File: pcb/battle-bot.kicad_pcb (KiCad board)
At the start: 4 copper layers, 82.1 x 54.4 mm, 229 parts, among them J1 Conn_01x01_Pin, J10 Conn_01x01_Pin, J11 Conn_01x01_Pin, J12 Conn_01x01_Pin, J13 Conn_ARM_SWD_TagConnect_TC203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, J3 Conn_01x01_Pin, J4 Conn_01x01_Pin, J5 Conn_01x01_Pin, J6 Conn_01x01_Pin, J7 Conn_01x01_Pin, J8 Conn_01x01_Pin, J9 Conn_01x01_Pin, Q1 AON7544, Q2 AO3401A, Q21 GANE3R9, Q22 GANE3R9, Q23 GANE3R9, Q24 GANE3R9, Q25 GANE3R9, Q26 GANE3R9, Q27 AON7544, Q28 AON7544, Q29 AON7544, Q30 AON7544, Q31 AON7544, Q32 AON7544, Q33 AON7544, Q34 AON7544, Q35 AON7544, Q36 AON7544, Q37 AON7544, Q38 AON7544, Q39 AON7544, Q40 AON7544, Q41 AON7544, Q42 AON7544, Q43 AON7544, U1 TPS53319, U10 LMG1205, U11 LMG1205, U12 LMG1205, U13 ACS780xLRTR-100B, U15 LP38690SD, U2 nRF24L01P, U3 AT2401C, U4 ICM-42688-P, U6 STM32G431RBTx, U7 DRV8323H, U8 DRV8323H, U9 DRV8323H, Y1 16MHz, Y2 16MHz

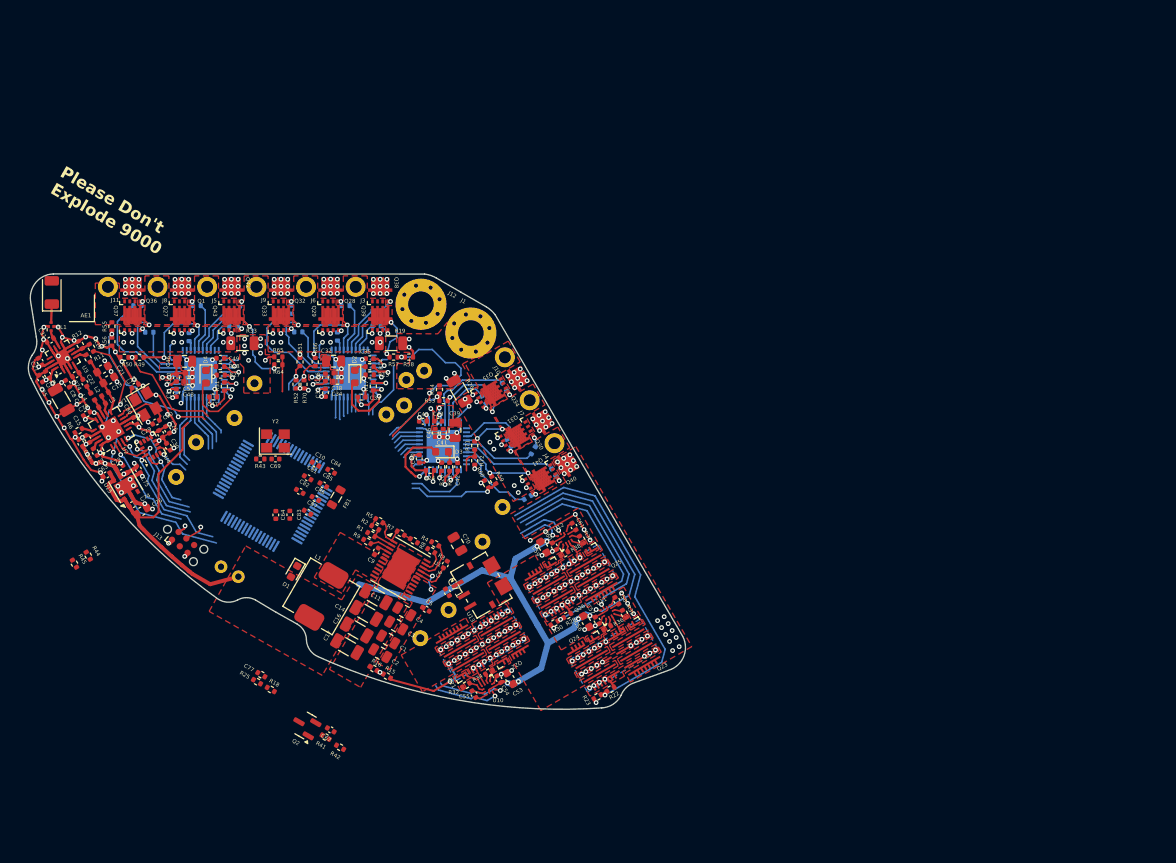
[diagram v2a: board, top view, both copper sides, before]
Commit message: Finish pcb
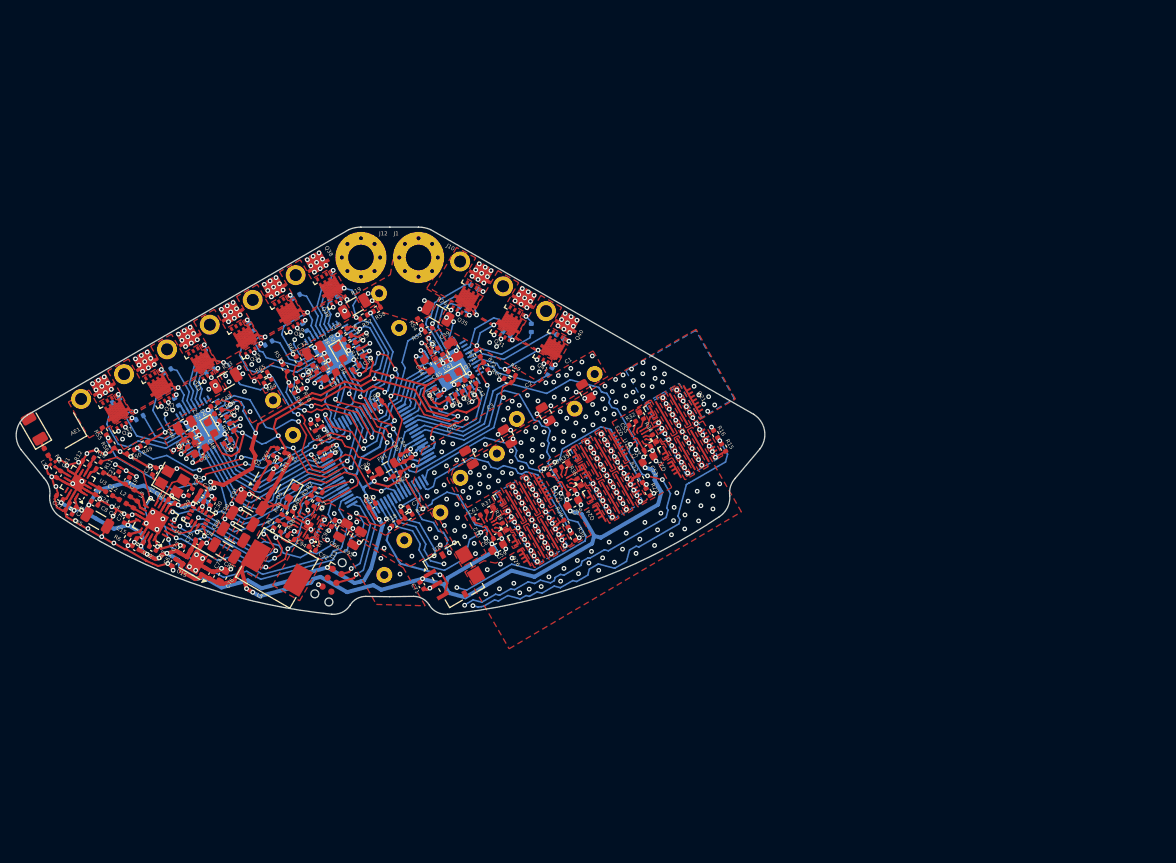
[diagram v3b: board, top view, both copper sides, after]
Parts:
- removed C11, C14, C16, C17: 47u, Capacitor_SMD:C_1206_3216Metric
- removed C18: 220u, Capacitor_THT:C_Radial_D6.3mm_H7.0mm_P2.50mm
- removed C4: 22u, Capacitor_SMD:C_0805_2012Metric
- removed C5, C6: 1u, Capacitor_SMD:C_0402_1005Metric
- removed C64, C69: 12p, Capacitor_SMD:C_0402_1005Metric
- removed C9: 100n, Capacitor_SMD:C_0402_1005Metric
- removed D1: LEDG, LED_SMD:LED_0603_1608Metric
- removed R4, R8: 100k, Resistor_SMD:R_0402_1005Metric
- removed R43, R9: 1k, Resistor_SMD:R_0402_1005Metric
- removed R5: 15k, Resistor_SMD:R_0402_1005Metric
- removed R7: 10k, Resistor_SMD:R_0402_1005Metric
- removed Y2: 16MHz, Crystal:Crystal_SMD_3225-4Pin_3.2x2.5mm
- added C88: 47u, Capacitor_SMD:C_1206_3216Metric, F.Cu at (72.5, 80.2)
- added C89: 47u, Capacitor_SMD:C_1206_3216Metric, F.Cu at (73.6, 78.2)
- added C90: 47u, Capacitor_SMD:C_1206_3216Metric, F.Cu at (74.8, 76.2)
- added C91: 47u, Capacitor_SMD:C_1206_3216Metric, F.Cu at (75.9, 74.2)
- added C92: 100n, Capacitor_SMD:C_0402_1005Metric, F.Cu at (83.5, 79.9)
- added C93: 100n, Capacitor_SMD:C_0402_1005Metric, F.Cu at (86.1, 76.8)
- added C94: 1u, Capacitor_SMD:C_0402_1005Metric, F.Cu at (80.8, 78.6)
- added C95: 22u, Capacitor_SMD:C_0805_2012Metric, F.Cu at (89.1, 78.6)
- added C96: 22u, Capacitor_SMD:C_0805_2012Metric, F.Cu at (87.3, 77.6)
- added D5: LEDW, LED_SMD:LED_0603_1608Metric, F.Cu at (80.9, 72.9)
- added L5: 2u2, Inductor_SMD:L_Chilisin_BMRB00060618, F.Cu at (79.1, 82.3)
- added R40: 33k, Resistor_SMD:R_0402_1005Metric, F.Cu at (79.9, 75.2)
- added R46: 4k7, Resistor_SMD:R_0402_1005Metric, F.Cu at (80.7, 75.7)
- added R47: 1k, Resistor_SMD:R_0402_1005Metric, F.Cu at (84.0, 74.2)
- added R48: 100k, Resistor_SMD:R_0402_1005Metric, F.Cu at (79.8, 77.4)
- C13: value 33n -> 100n
- C19, C21: footprint Capacitor_SMD:C_0603_1608Metric -> Capacitor_SMD:C_0402_1005Metric
- C37, C44, C51: footprint Capacitor_SMD:C_0402_1005Metric -> Capacitor_SMD:C_0603_1608Metric
- C73: value 2u2 -> 10u
- L1: value 1u -> 6n8; footprint Inductor_SMD:L_Changjiang_FXL0630 -> Inductor_SMD:L_0402_1005Metric
- R1: value 47k -> 4k7
- R2: value 4k7 -> 51k
- R3: value 100k -> 4k7
- U1: value TPS53319 -> TPS56C230; footprint Package_DFN_QFN:DFN-22-1EP_5x6mm_P0.5mm_EP3.14x4.3mm -> User_Footprints:VQFN-20_3x3mm_P0.45
- moved R16 51.8 mm to (133.9, 65.6), turned to 120 degrees
- moved R15 50.9 mm to (134.9, 67.3), turned to -60 degrees
- moved R32 40.2 mm to (124.6, 63.3), turned to 120 degrees
- moved Q21 40.1 mm to (128.8, 62.8), turned to 30 degrees
- moved C1 39.7 mm to (117.7, 60.3), turned to 120 degrees
- moved C55 39.2 mm to (123.5, 64.3), turned to -150 degrees
- moved L1 38.9 mm to (50.2, 67.8), turned to 120 degrees
- moved R42 37.8 mm to (79.6, 67.7)
- moved U10 36.5 mm to (124.3, 66.1), turned to -150 degrees
- moved C2 36.3 mm to (112.6, 63.2), turned to 120 degrees
- moved R34 35.8 mm to (126.3, 66.2), turned to -60 degrees
- moved R45 35.4 mm to (84.5, 64.2), turned to 120 degrees
- moved R41 34.8 mm to (79.2, 69.2), turned to 60 degrees
- moved C67 34.7 mm to (78.4, 68.7), turned to 60 degrees
- moved C54 34.3 mm to (125.4, 67.4), turned to 30 degrees
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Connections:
- C65 pad 1: GND -> VDD
- C65 pad 2: VDD -> GND
- C66 pad 1: VDD -> GND
- C66 pad 2: GND -> VDD
- C68 pad 1: GND -> VDD
- C68 pad 2: VDD -> GND
- C72 pad 1: GND -> VDD
- C72 pad 2: VDD -> GND
- FL1 pad 2: Net-(AE1-FEED) -> Net-(FL1-OUT)
- L1 pad 1: Net-(C9-Pad1) -> Net-(FL1-OUT)
- L1 pad 2: +5V -> Net-(AE1-FEED)
- R1 pad 1: /REN -> Net-(U1-MODE)
- R1 pad 2: VDD -> GND
- R2 pad 1: GND -> VDD
- R2 pad 2: /REN -> /EN
- R3 pad 1: Net-(U1-TRIP) -> /EN
- U1 pad 10: Net-(C9-Pad1) -> GND
- U1 pad 11: Net-(C9-Pad1) -> unconnected-(U1-SS-Pad11)
- U1 pad 12: VDD -> /EN
- U1 pad 13: VDD -> GND
- U1 pad 14: VDD -> Net-(U1-FB)
- U1 pad 15: VDD -> Net-(U1-MODE)
- U1 pad 16: VDD -> GND
- U1 pad 17: VDD -> Net-(U1-VCC)
- U1 pad 18: Net-(U1-VREG) -> GND
- U1 pad 19: VDD -> Net-(C92-Pad1)
- U1 pad 2: /REN -> VDD
- U1 pad 20: Net-(U1-MODE) -> Net-(C92-Pad1)
- U1 pad 21: Net-(U1-TRIP) -> GND
- U1 pad 3: /PGD -> VDD
- U1 pad 4: Net-(U1-VBST) -> VDD
- U1 pad 5: GND -> VDD
- U1 pad 6: Net-(C9-Pad1) -> Net-(C92-Pad1)
- U1 pad 7: Net-(C9-Pad1) -> GND
- U1 pad 8: Net-(C9-Pad1) -> GND
- U1 pad 9: Net-(C9-Pad1) -> /PGD
- U6 pad 10: /WHC -> /CPC1
- U6 pad 11: /CPB3 -> /CPB1
- U6 pad 12: /SO1 -> /CPC2
- U6 pad 13: /SO2 -> /SO1
- U6 pad 14: /SO3 -> /CPA1
- U6 pad 17: /WSO -> /INHC2
- U6 pad 18: /WCPA -> /INLB2
- U6 pad 19: /WCPB -> /INHB2
- U6 pad 2: /WLA -> /INLC2
- U6 pad 20: /WCPC -> /INLA2
- U6 pad 21: /CPA2 -> /SO2
- U6 pad 23: /CPC2 -> /WLC
- U6 pad 24: /WLB -> /WLA
- U6 pad 25: /WLC -> /WLB
- U6 pad 26: /CPA3 -> /CPA2
- U6 pad 3: /GINT -> /INLC1
- U6 pad 30: /INHC1 -> /INHA2
- U6 pad 33: /CPC3 -> /WCPB
- U6 pad 34: /CPA1 -> /WCPC
- U6 pad 35: /CLK -> unconnected-(U6-PB13-Pad35)
- U6 pad 36: /CPB1 -> /WCPA
- U6 pad 37: /CPC1 -> /WSO
- U6 pad 38: /INHA2 -> /INHA1
- U6 pad 39: /INHB2 -> /INHB1
- U6 pad 4: /INLB3 -> /INLB1
- U6 pad 40: /INHC2 -> /INHC1
- U6 pad 41: /INLA1 -> /INHA3
- U6 pad 42: /RCS -> unconnected-(U6-PA8-Pad42)
- U6 pad 43: /GCS -> /WHA
- U6 pad 44: /MISO -> /WHB
- U6 pad 45: /MOSI -> /WHC
- U6 pad 5: /XTO -> /CPC3
- U6 pad 51: /INLC3 -> /RCS
- U6 pad 52: /INLB2 -> /CLK
- U6 pad 53: /INLC1 -> /MISO
- U6 pad 54: /INLC2 -> /MOSI
- U6 pad 55: /INLA3 -> /GCS
- U6 pad 56: /INHB1 -> /RIRQ
- U6 pad 57: /INLA2 -> /GINT
- U6 pad 58: /INHA1 -> /INLC3
- U6 pad 59: /INHA3 -> /INHC3
- U6 pad 6: /XTI -> /CPA3
- U6 pad 60: /INHB3 -> /INLB3
- U6 pad 61: /INHC3 -> /INHB3
- U6 pad 62: /INLB1 -> /INLA3
- U6 pad 7: /RIRQ -> /INLA1
- U6 pad 8: /WHA -> /SO3
- U6 pad 9: /WHB -> /CPB3
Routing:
- net +3V3: track 89.0 -> 223.0 mm, vias 19 -> 27
- net /WCPA: track 0.98 -> 63.7 mm, vias 1 -> 3
- net /CAL: track 4.31 -> 59.8 mm, vias 0 -> 6
- net +5V: track 131.2 -> 186.7 mm, vias 9 -> 15
- net /WHA: track 8.77 -> 59.4 mm, vias 1 -> 5
- net /WLA: track 8.80 -> 38.5 mm
- net /SO3: track 1.94 -> 30.3 mm, vias 0 -> 2
- net /CPB3: track 14.2 -> 38.9 mm, vias 1 -> 5
- net /RIRQ: track 0.00 -> 24.4 mm, vias 0 -> 1
- net /INHA3: track 5.19 -> 29.3 mm, vias 0 -> 2
- net /WLC: track 5.77 -> 24.7 mm, vias 1 -> 3
- net /INLC2: track 3.76 -> 22.5 mm, vias 0 -> 2
- net /RCE: track 36.2 -> 54.7 mm, vias 2 -> 4
- net /RCS: track 13.2 -> 31.6 mm
- net /CPC3: track 19.6 -> 37.1 mm, vias 2 -> 3
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- added copper zone on In1.Cu, net /LargeMotor/LargeBridgeA/PL
- added copper zone on F.Cu, net Net-(C92-Pad1)
- added copper zone on B.Cu, net VDD
- removed copper zone on F.Cu, net Net-(C9-Pad1)
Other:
- board size 82.1 x 54.4 mm -> 93.6 x 48.4 mm
- board text added: "Made By Miguel Flores-Acton"
